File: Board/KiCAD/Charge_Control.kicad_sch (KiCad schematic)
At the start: 57 parts, among them Q1 AON7408, Q10 AON7407, Q2 AON7408, Q3 AON7408, Q4 AON7408, U1 BQ25730RSNR, U3 LTC2943CDD#PBF

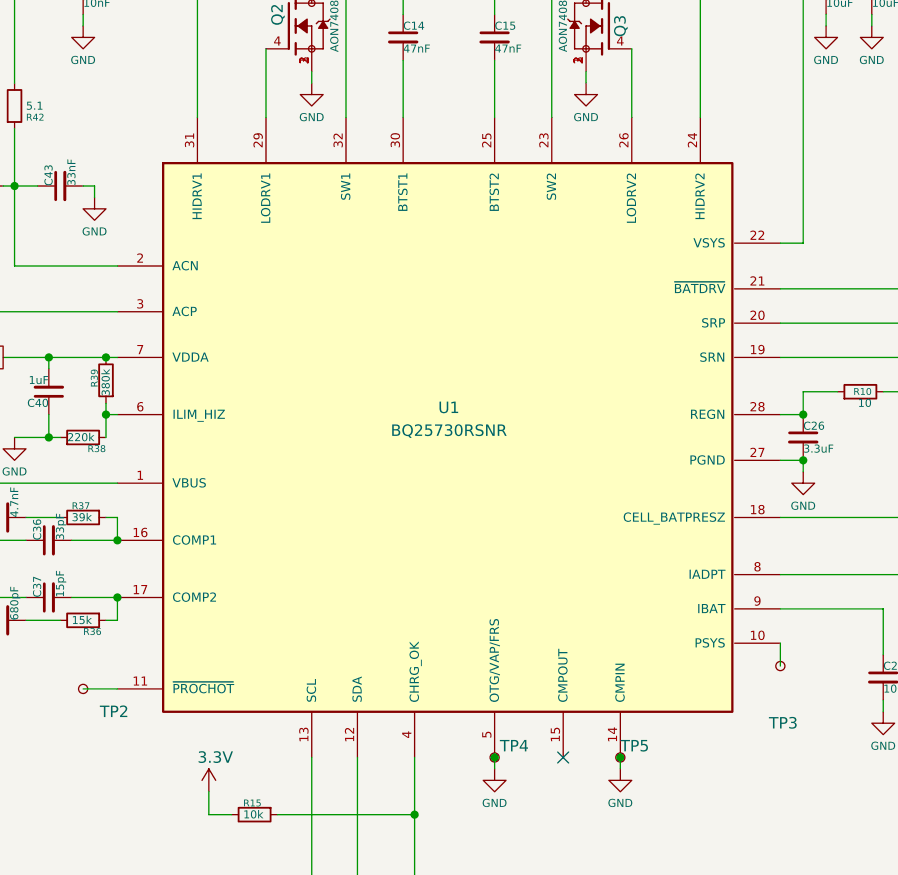
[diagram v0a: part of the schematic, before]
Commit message: Edits to PCB
@andrewgreenberg @KeytarGoblin
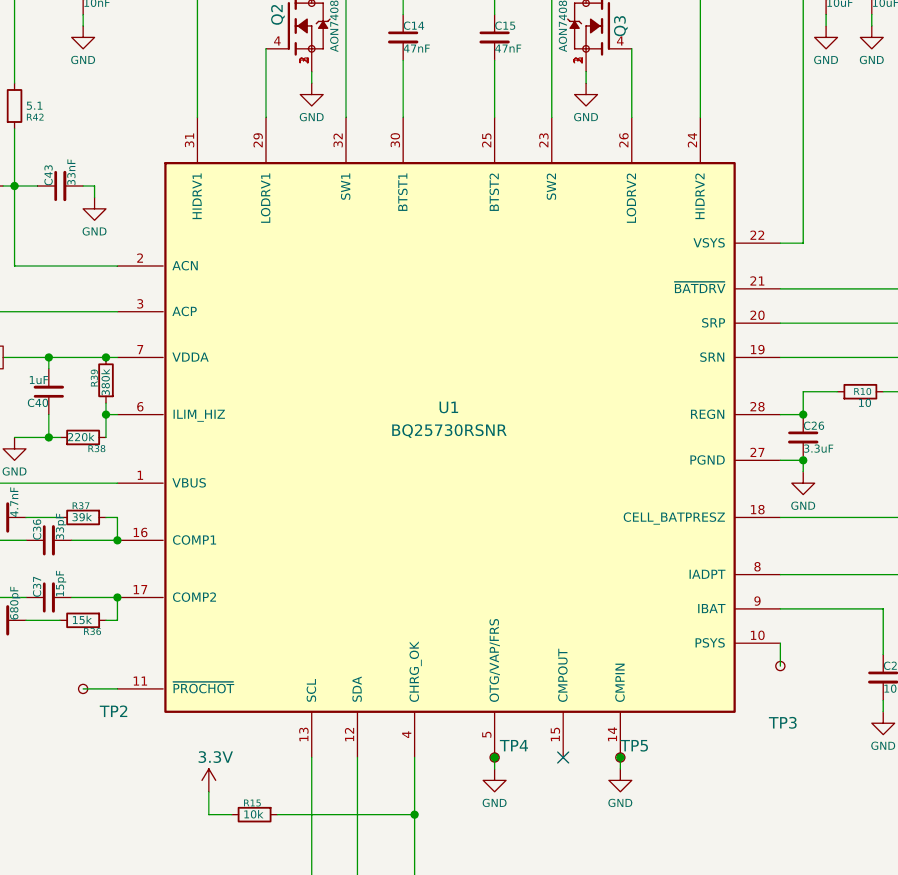
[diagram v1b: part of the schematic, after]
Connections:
- net GND renamed 33
- net 33: now also U1.33, U1.34, U1.35, U1.36, U1.37, U1.38, U1.39, U1.40, U1.41, U1.42
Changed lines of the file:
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@@
 	)
 	(symbol
-		(lib_name "BQ25730RSNR_1")
 		(lib_id "BQ25730RSNR:BQ25730RSNR")
 		(at 123.19 88.9 0)
@@
 		(pin "27"
 		)
+		(pin "39"
+		)
+		(pin "33"
+		)
+		(pin "40"
+		)
+		(pin "35"
+		)
+		(pin "38"
+		)
+		(pin "36"
+		)
+		(pin "41"
+		)
+		(pin "34"
+		)
+		(pin "37"
+		)
+		(pin "42"
+		)
 		(instances
